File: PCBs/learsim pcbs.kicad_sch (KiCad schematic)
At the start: 56 parts, among them SW1 MHz, SW2 KHz, SW3 2MD1T1B1M2QES-5, U1 ESP32-C6-DEV-KIT-N8, U2 MAX7219, U3 MAX7219

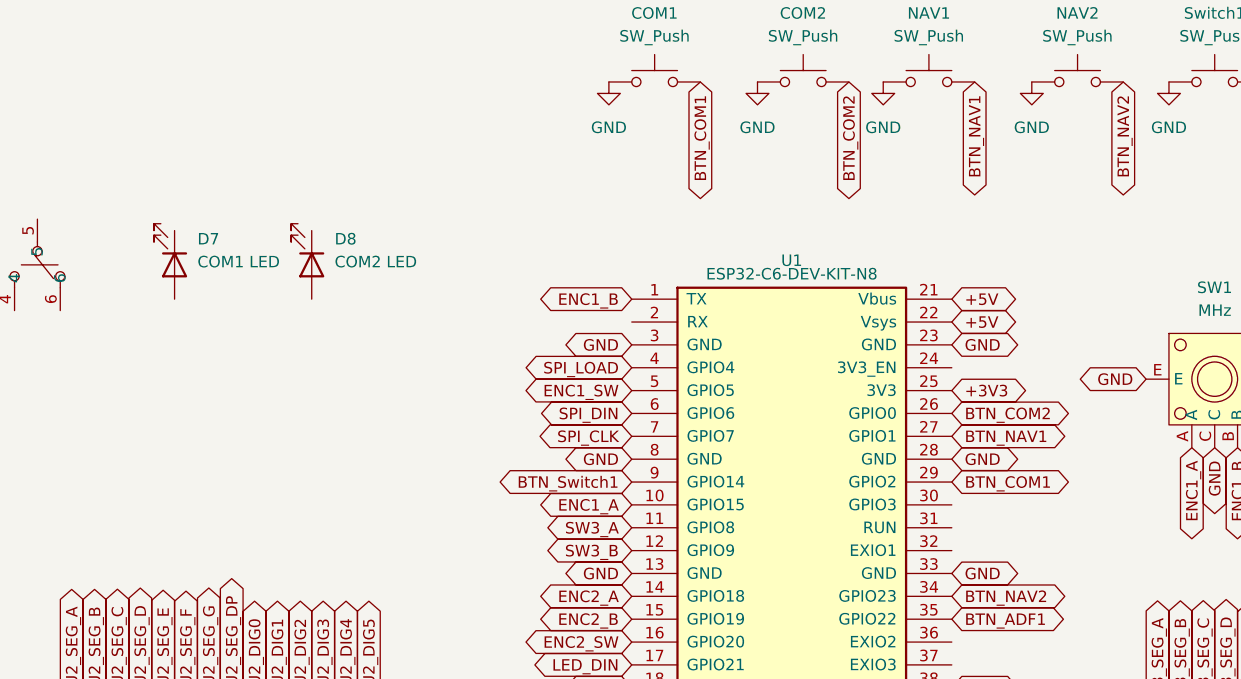
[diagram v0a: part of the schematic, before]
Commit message: Update drill files and job configuration with new creation timestamps and modified drill sizes
- Updated creation timestamps in NPTH and PTH drill files to 2026-07-26T23:00:48.
- Adjusted drill sizes for T4, T5, and T6 in the PTH drill file.
- Added new coordinates in the PTH drill file for improved component placement.
- Updated creation date in the job configuration file to 2026-07-26T23:00:53.
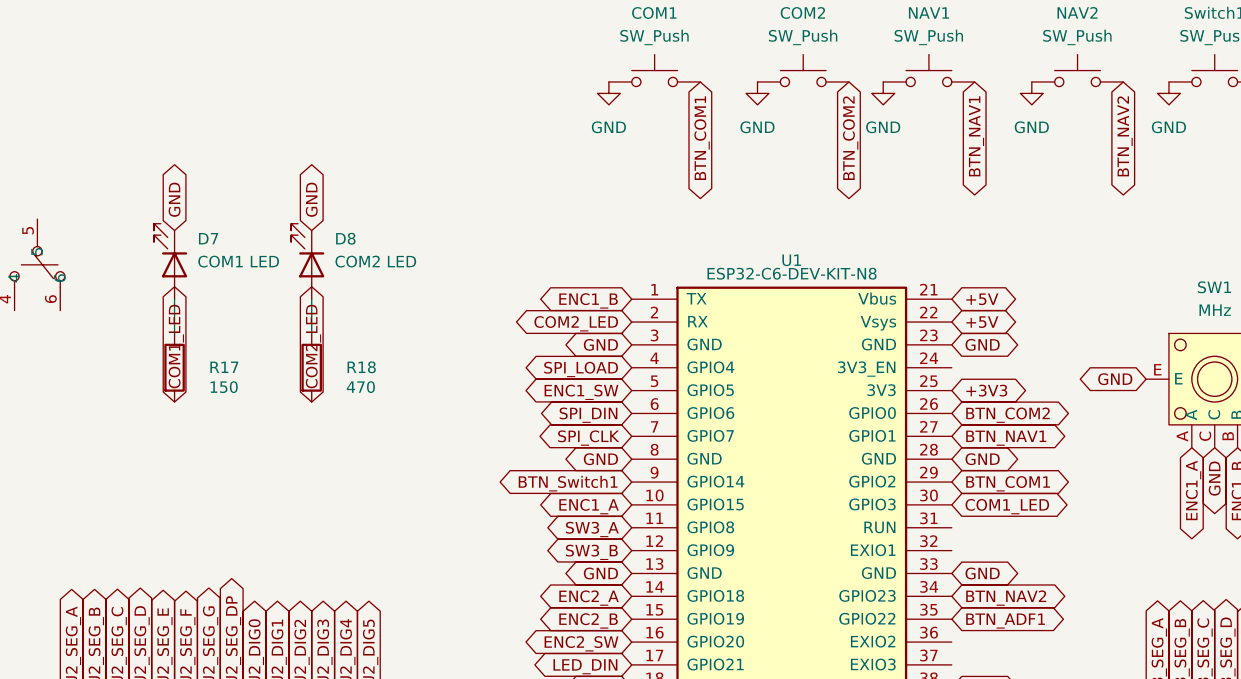
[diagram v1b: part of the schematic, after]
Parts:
- added R17: 150, Resistor_THT:R_Axial_DIN0207_L6.3mm_D2.5mm_P7.62mm_Horizontal, symbol Device:R
- added R18: 470, Resistor_THT:R_Axial_DIN0207_L6.3mm_D2.5mm_P7.62mm_Horizontal, symbol Device:R
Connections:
- net GND: now also D7.1 (K), D8.1 (K)
- net COM2_LED: now reaches U1.2 (RX)
- net COM2_LED: now also R18.2
- net COM1_LED: now reaches U1.30 (GPIO3)
- net COM1_LED: now also R17.2
- net at D8.2 (A): now also R18.1
- net at D7.2 (A): now also R17.1
